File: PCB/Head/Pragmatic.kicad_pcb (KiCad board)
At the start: 2 copper layers, 11 parts, among them J1 Conn_02x07_Odd_Even, J2 Conn_02x07_Odd_Even, SW1 SW_Push, SW2 SW_Push, SW3 SW_Push, SW4 SW_Push, U1 ProMicro

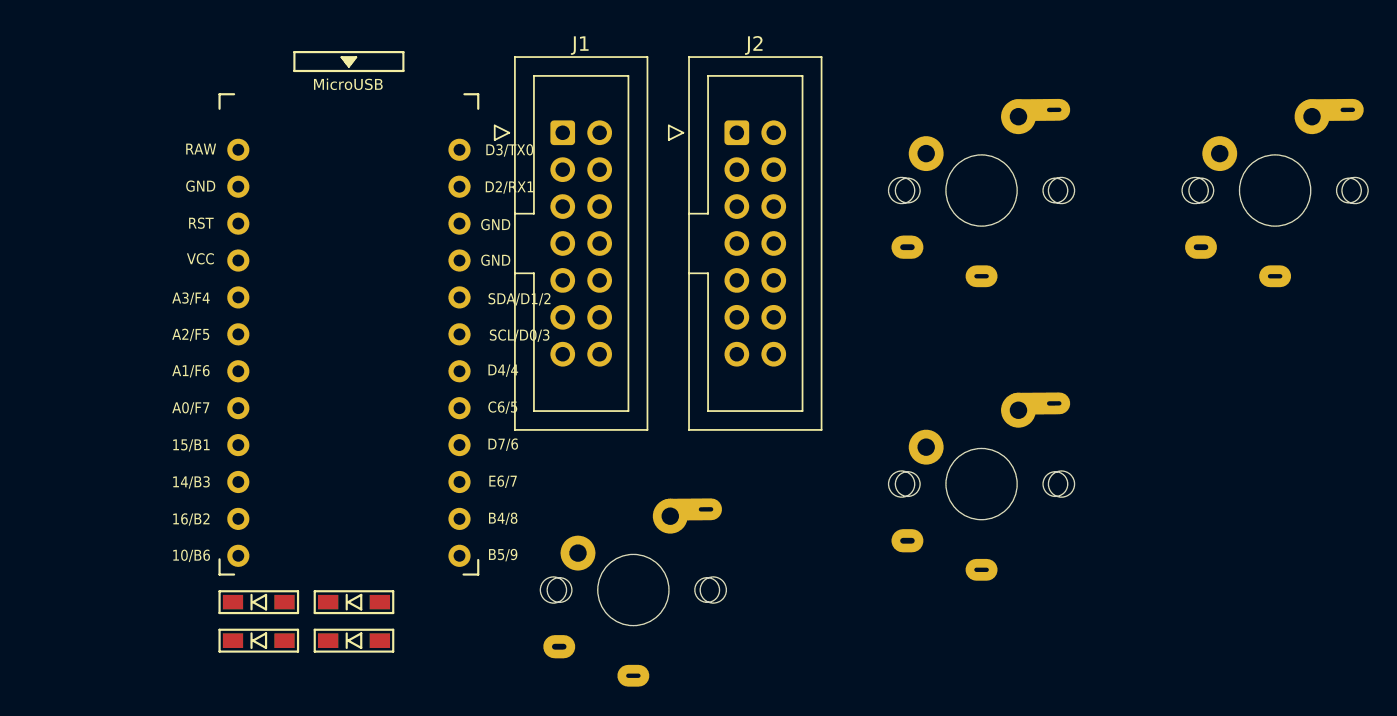
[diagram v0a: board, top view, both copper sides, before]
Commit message: head board
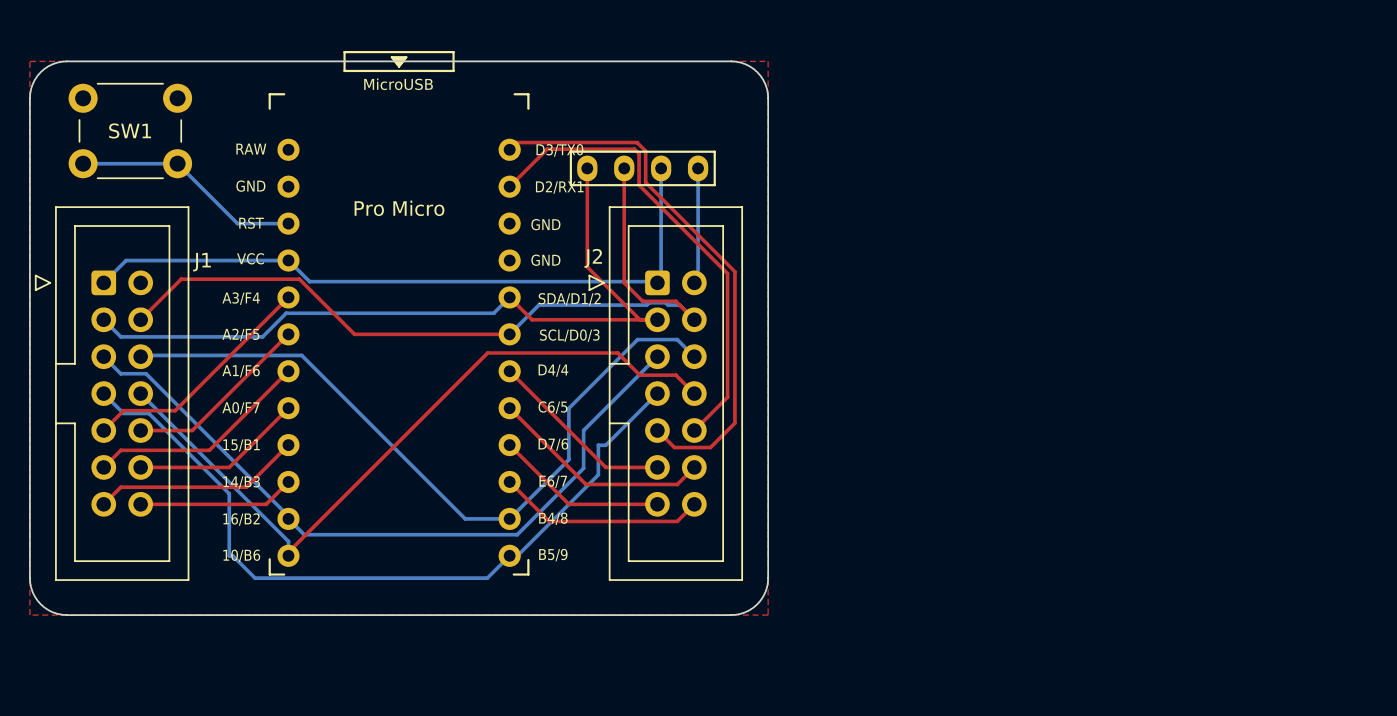
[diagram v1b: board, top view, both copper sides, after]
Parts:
- removed D1, D2, D3, D4: D, Foostan:D3_SMD_v2
- removed SW2, SW3, SW4: SW_Push, Foostan:CherryMX_ChocV2_1u
- added J3: I2C connector, Foostan:OLED_1side, F.Cu at (160.3, 50.5)
- J1: value Conn_02x07_Odd_Even -> Left
- J2: value Conn_02x07_Odd_Even -> Right
- SW1: footprint Foostan:CherryMX_ChocV2_1u -> Button_Switch_THT:SW_PUSH_6mm
- moved SW1 42.9 mm to (124.5, 50.2), turned to 180 degrees
- moved J1 33.2 mm to (119.4, 58.4)
- moved J2 11.7 mm to (157.5, 58.4)
- moved U1 3.45 mm to (139.7, 63.7)
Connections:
- J1 pad 10: Col3 -> Col2
- J1 pad 11: Row4 -> Col3
- J1 pad 13: Col6 -> Col5
- J1 pad 14: Col5 -> Col6
- J1 pad 4: Col1 -> Row2
- J1 pad 6: Col1 -> Row4
- J1 pad 7: Row6 -> Row5
- J1 pad 8: Col1 -> Row6
- J1 pad 9: Row5 -> Col1
- J2 pad 10: (no net) -> Col8
- J2 pad 11: (no net) -> Col9
- J2 pad 12: (no net) -> Col10
- J2 pad 13: (no net) -> Col11
- J2 pad 14: (no net) -> Col12
- J2 pad 4: Col7 -> Row2
- J2 pad 5: Col1 -> Row3
- J2 pad 6: Col8 -> Row4
- J2 pad 7: Row3 -> Row5
- J2 pad 8: Col9 -> Row6
- J2 pad 9: (no net) -> Col7
- SW1 pad 1: Net-(D1-Pad2) -> Reset
- SW1 pad 2: Col1 -> Ground
- U1 pad 1: Col1 -> Col7
- U1 pad 10: Col6 -> Col12
- U1 pad 11: Row3 -> Row4
- U1 pad 12: Row4 -> Row5
- U1 pad 14: Row5 -> Row3
- U1 pad 15: Col7 -> Col6
- U1 pad 16: Col8 -> Col5
- U1 pad 17: Col9 -> Col4
- U1 pad 18: (no net) -> Col3
- U1 pad 19: (no net) -> Col2
- U1 pad 2: Col1 -> Col8
- U1 pad 20: (no net) -> Col1
- U1 pad 22: (no net) -> Reset
- U1 pad 24: (no net) -> Net-(U1-Pad24)
- U1 pad 6: Col1 -> Row2
- U1 pad 7: Col3 -> Col9
- U1 pad 8: Col4 -> Col10
- U1 pad 9: Col5 -> Col11
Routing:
- net Row2: track 0.00 -> 56.0 mm
- net Row1: track 0.00 -> 53.5 mm
- net Row5: track 0.00 -> 52.3 mm
- net Row4: track 0.00 -> 50.5 mm
- net Row6: track 0.00 -> 50.4 mm
- net Row3: track 0.00 -> 49.9 mm
- net VCC: track 0.00 -> 47.4 mm
- net Col7: track 0.00 -> 37.6 mm
- net Col8: track 0.00 -> 32.6 mm
- net Col1: track 0.00 -> 16.5 mm
- net Reset: track 0.00 -> 15.8 mm
- net Col3: track 0.00 -> 15.5 mm
- net Col10: track 0.00 -> 15.4 mm
- net Col5: track 0.00 -> 14.4 mm
- net Col12: track 0.00 -> 14.3 mm
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- added copper zone on F.Cu, net Ground
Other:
- board outline added: 50.8 x 38.1 mm
- board text added: "Pragmatic"
- board text added: "Pragmatic - Brain v1 James Sa 2021-11-07"
